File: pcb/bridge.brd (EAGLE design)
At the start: 104.2 x 63.6 mm, 38 parts, among them IC2 LM358D, IC3 78L05SMD, X1 PN61729-S

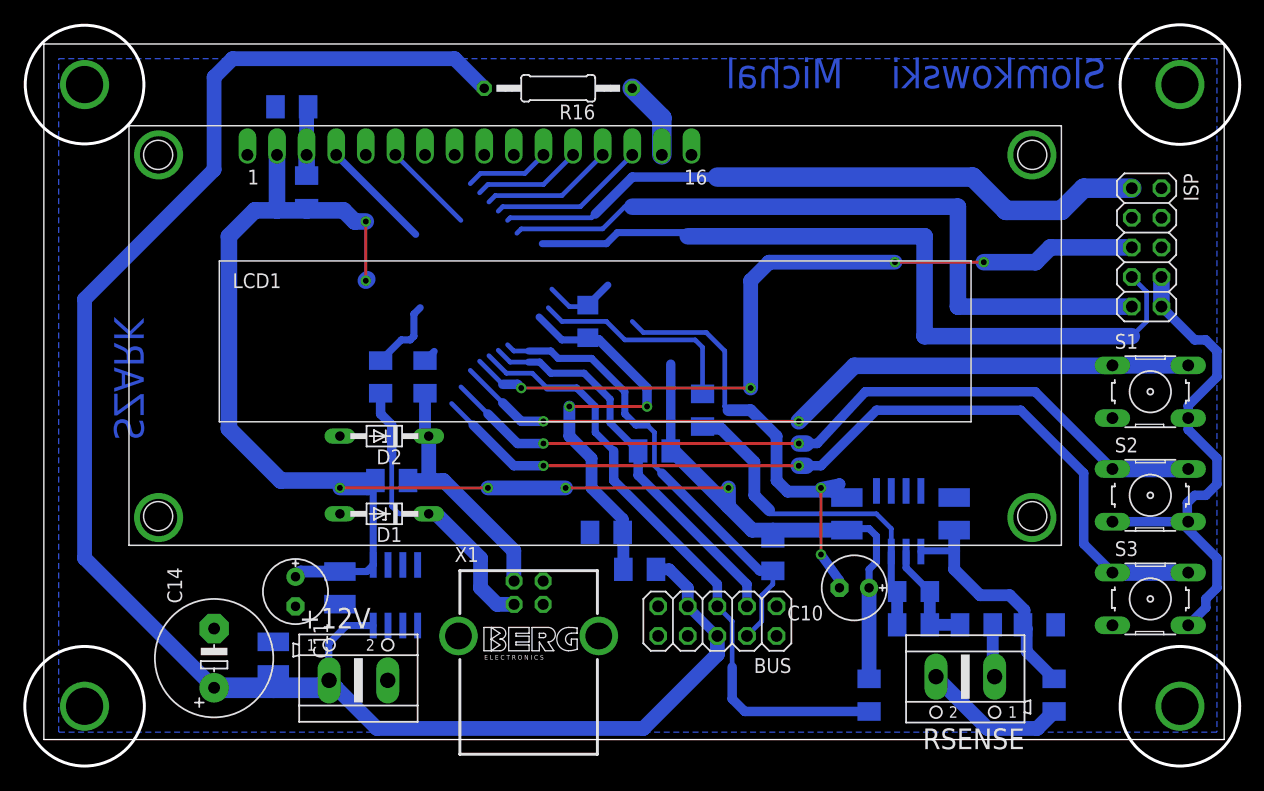
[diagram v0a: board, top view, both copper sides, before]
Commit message: bridge: Schematic beta version.
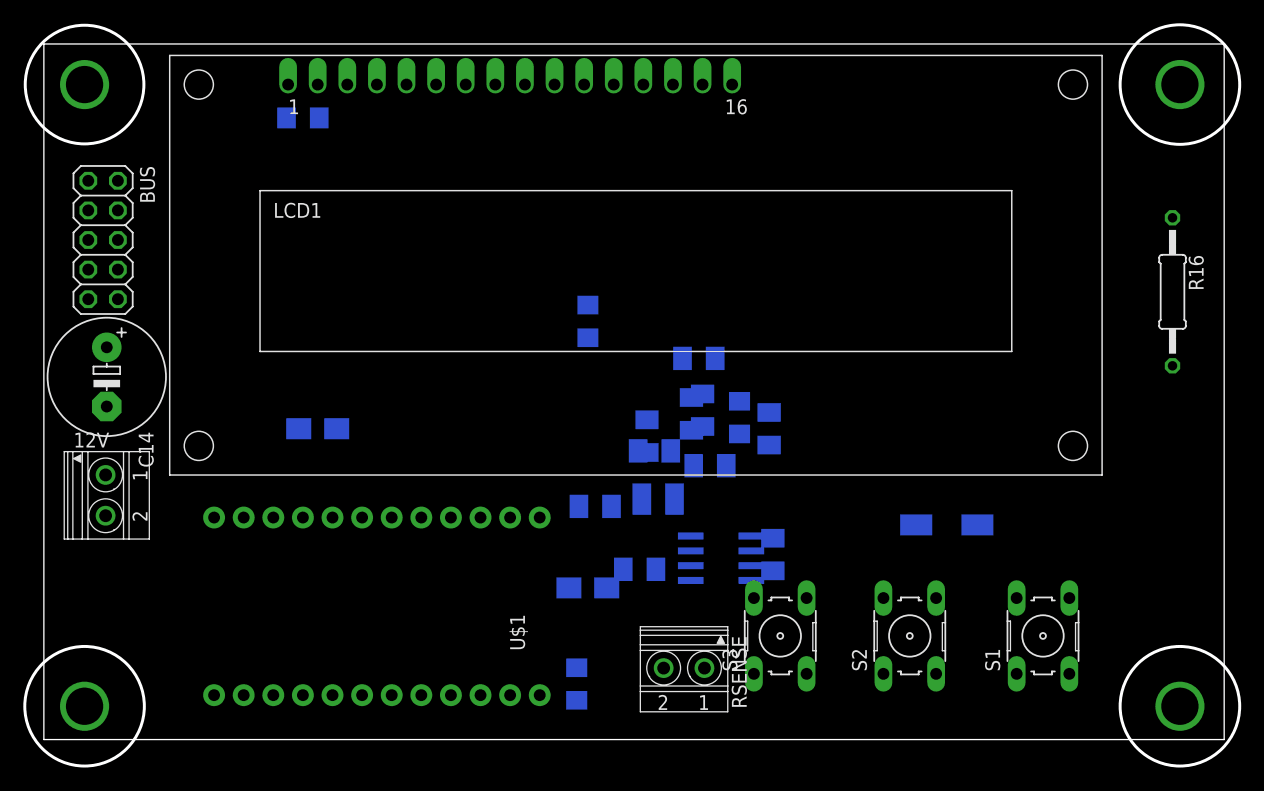
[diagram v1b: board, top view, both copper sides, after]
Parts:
- removed +12V: (no value), con-ptr500:AK500/2
- removed C10, C11: 22u, rcl:E2,5-6E
- removed C12, C13, C9: 100n, rcl:C1210
- removed D1, D2: 3V6, diode:DO34Z7
- removed IC3: 78L05SMD, linear:SO08
- removed ISP: (no value), pinhead:2X05
- removed R11, R12: 68, rcl:M1206
- removed R13: 1k5, rcl:M1206
- removed R14: 10k, rcl:M1206
- removed R15: 1k, rcl:M1206
- removed X1: PN61729-S, con-berg:PN61729-S
- added 12V: (no value), con-phoenix-350:1751248
- added C1, C2: 4u7, rcl:B/3528-21W
- added C3, C4: 100n, rcl:C1206
- added C5: 47u, rcl:C/6032-28W
- added U$1: ARDUINO_PRO_MICRO, sparkfun-boards:ARDUINO_PRO_MICRO
- RSENSE: device con-ptr500:AK500/2 -> con-phoenix-350:1751248
- moved BUS 62.0 mm to (4.76, 43.8), turned to 270 degrees
- moved R16 55.5 mm to (96.5, 39.4), turned to 270 degrees
- moved R4 37.3 mm to (51.4, 27.0), turned to 270 degrees
- moved R3 35.5 mm to (56.8, 24.4), turned to 0 degrees
- moved R8 32.4 mm to (55.9, 33.7), turned to 0 degrees
- moved S3 31.9 mm to (62.9, 9.84), turned to 90 degrees
- moved R6 26.3 mm to (55.2, 28.9), turned to 270 degrees
- moved C14 25.8 mm to (5.08, 32.1), turned to 270 degrees
- moved C7 25.4 mm to (52.4, 21.6), turned to 180 degrees
- moved R5 24.5 mm to (61.9, 27.6), turned to 270 degrees
- moved RSENSE 24.1 mm to (54.6, 6.99)
- moved S2 23.9 mm to (74.0, 9.84), turned to 90 degrees
- moved S1 22.9 mm to (85.4, 9.84), turned to 90 degrees
- moved C8 21.1 mm to (59.4, 28.6), turned to 90 degrees
- moved IC2 15.6 mm to (57.8, 16.5), turned to 90 degrees
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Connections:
- removed net N$3: LCD1.3, R14.1, R15.2
- removed net N$5: D2.C, R11.2, R13.1, X1.2
- removed net N$6: D1.C, R12.2, X1.3
- removed net PB0: LCD1.12
- removed net PB1: LCD1.13
- removed net PB2: LCD1.14
- removed net PB3: ISP.1
- removed net PB4: ISP.9
- removed net PB5: ISP.7
- removed net PC0: R7.2
- removed net PC1: C6.1, R1.1, R2.2
- removed net PC3: BUS.4, R10.1
- removed net PC4: BUS.3, R9.1
- removed net PC5: BUS.5, R8.1
- removed net PD0: S1.1, S1.2
- removed net PD1: S2.1, S2.2
- removed net PD2: S3.1, S3.2
- removed net PD3: R11.1
- removed net PD4: R12.1
- removed net PD5: LCD1.4
- removed net PD6: LCD1.6
- removed net PD7: LCD1.11
- removed net RESET: ISP.5
- new net ACURR: C2.+, C3.1, R7.2, U$1.12
- new net AVLTG: C1.+, C6.1, R1.1, R2.2, U$1.20
- new net BTN1: S3.1, S3.2, U$1.9
- new net BTN2: S2.1, S2.2, U$1.10
- new net BTN3: S1.1, S1.2, U$1.11
- new net DDB4: LCD1.11, U$1.16
- new net DDB5: LCD1.12, U$1.15
- new net DDB6: LCD1.13, U$1.14
- new net DDB7: LCD1.14, U$1.13
- new net DE: LCD1.6, U$1.17
- new net DRS: LCD1.4, U$1.19
- new net DRW: LCD1.5, U$1.18
- new net RX: U$1.2
- new net SCL: BUS.5, R8.1, U$1.6
- new net SDA: BUS.3, R9.1, U$1.5
- new net STOP: BUS.4, R10.1, U$1.7
- new net TX: U$1.1
- net +12V: now also 12V.1, U$1.24; no longer +12V.1, C13.2, IC3.8
- net +5V: now also C4.1, C5.+, U$1.21; no longer C10.+, C11.+, C12.2, C9.2, IC3.1, R13.2, R14.2
- net GND: now also 12V.2, C1.-, C2.-, C3.2, C4.2, C5.-, LCD1.3, U$1.23, U$1.3, U$1.4; no longer +12V.2, C10.-, C11.-, C12.1, C13.1, C9.1, D1.A, D2.A, IC3.2, IC3.3, IC3.6, IC3.7, ISP.10, ISP.4, ISP.6, ISP.8, LCD1.5, R15.1, X1.4, X1.S1, X1.S2
- net N$21: now also RSENSE.2; no longer RSENSE.1
- net N$29: now also RSENSE.1; no longer RSENSE.2
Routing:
- net +12V: track 153.2 -> 0.00 mm
- net +5V: track 148.3 -> 0.00 mm, vias 6 -> 0
- net GND: track 91.7 -> 0.00 mm, vias 2 -> 0
- net PD2: track 76.7 -> 0.00 mm, vias 2 -> 0
- net PD1: track 69.7 -> 0.00 mm, vias 2 -> 0
- net RESET: track 67.3 -> 0.00 mm, vias 4 -> 0
- net PB5: track 66.0 -> 0.00 mm
- net PD0: track 65.4 -> 0.00 mm, vias 2 -> 0
- net PB4: track 62.3 -> 0.00 mm
- net PB3: track 57.1 -> 0.00 mm
- net PC5: track 53.1 -> 0.00 mm
- net PC3: track 40.1 -> 0.00 mm
- net PC1: track 36.2 -> 0.00 mm, vias 2 -> 0
- net PC4: track 34.0 -> 0.00 mm
- net NET3: track 30.1 -> 0.00 mm
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- removed copper zone on layer 16, net GND
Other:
- board text removed: "Michal"
- board text removed: "SZARK"
- board text removed: "Slomkowski"
